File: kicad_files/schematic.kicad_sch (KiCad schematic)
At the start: 54 parts, among them J1 USB_C_Receptacle_USB2.0_14P, J2 Barrel_Jack, Q1 MMBT3904, SW1 SW_Push, SW2 RST, SW3 BOOT, U1 ESP32-C3-WROOM-02, U2 TPS5430DDA, U3 AMS1117-3.3

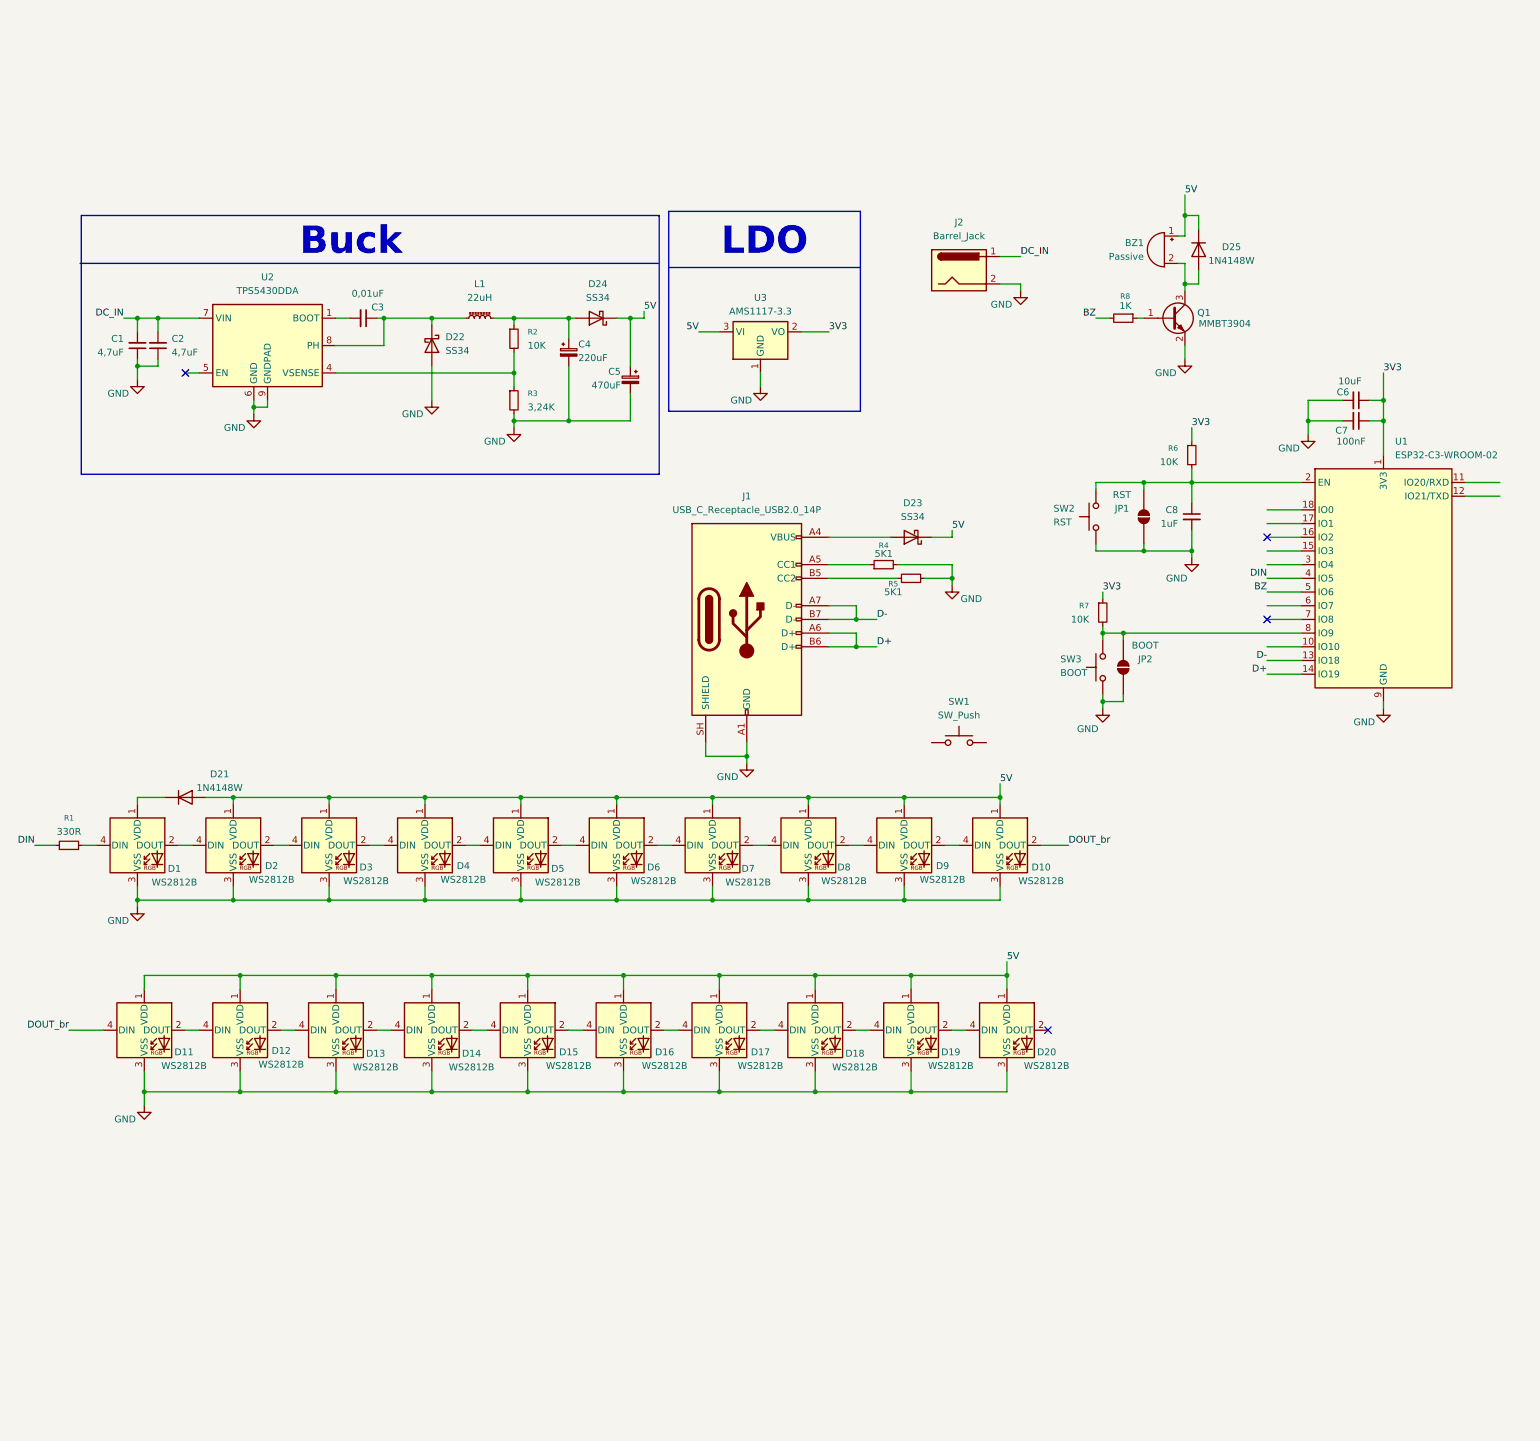
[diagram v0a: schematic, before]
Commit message: Add files via upload
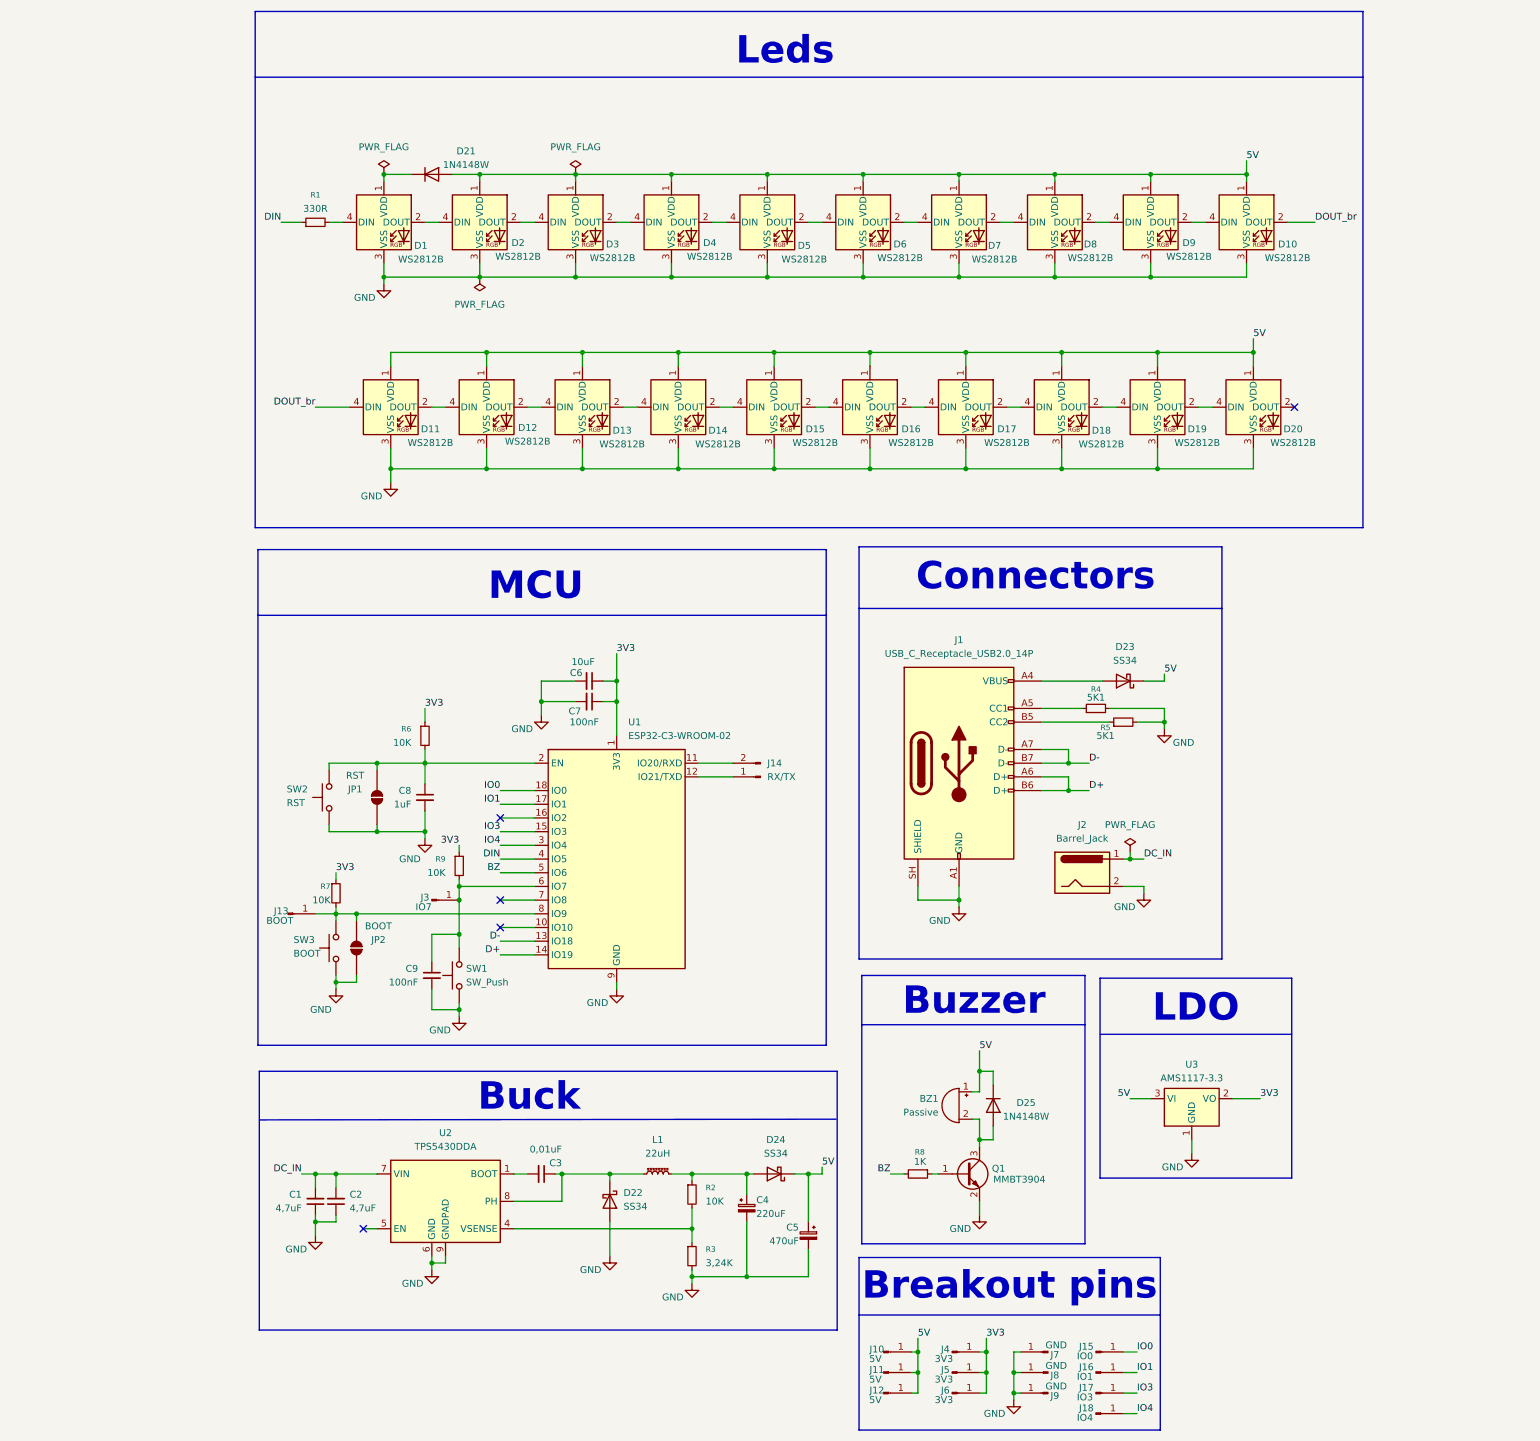
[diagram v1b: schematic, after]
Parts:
- added C9: 100nF, symbol Device:C_Small
- added J10, J11, J12: 5V, symbol Connector:Conn_01x01_Pin
- added J13: BOOT, symbol Connector:Conn_01x01_Pin
- added J14: RX/TX, symbol Connector:Conn_01x02_Pin
- added J15: IO0, symbol Connector:Conn_01x01_Pin
- added J16: IO1, symbol Connector:Conn_01x01_Pin
- added J17: IO3, symbol Connector:Conn_01x01_Pin
- added J18: IO4, symbol Connector:Conn_01x01_Pin
- added J3: IO7, symbol Connector:Conn_01x01_Pin
- added J4, J5, J6: 3V3, symbol Connector:Conn_01x01_Pin
- added J7, J8, J9: GND, symbol Connector:Conn_01x01_Pin
- added R9: 10K, symbol Device:R_Small
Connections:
- net 3V3: now also J4.1 (Pin_1), J5.1 (Pin_1), J6.1 (Pin_1), R9.1
- net 5V: now also J10.1 (Pin_1), J11.1 (Pin_1), J12.1 (Pin_1)
- net GND: now also SW1.1, C9.2, J7.1 (Pin_1), J8.1 (Pin_1), J9.1 (Pin_1)
- net at U1.11 (IO20/RXD): now also J14.2 (Pin_2)
- net at U1.12 (IO21/TXD): now also J14.1 (Pin_1)
- net IO3: now reaches U1.15 (IO3)
- net IO3: now also J17.1 (Pin_1)
- net IO1: now reaches U1.17 (IO1)
- net IO1: now also J16.1 (Pin_1)
- net IO0: now reaches U1.18 (IO0)
- net IO0: now also J15.1 (Pin_1)
- net IO4: now reaches U1.3 (IO4)
- net IO4: now also J18.1 (Pin_1)
- net at U1.6 (IO7): now also SW1.2, C9.1, J3.1 (Pin_1), R9.2
- net at JP2.1 (A), R7.2, SW3.2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: now also J13.1 (Pin_1)
- no-connect marks 4 -> 5
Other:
- note added: "Breakout pins"
- note added: "Buzzer"
- note added: "Connectors"
- note added: "Leds"
- note added: "MCU"
- moved on the sheet: BZ1, C1, C2, C3, C4, C5, C6, C7, C8, D1, D10, D11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
